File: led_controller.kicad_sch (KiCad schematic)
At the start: 33 parts, among them IC1 ESP32-C3-MINI-1-N4X, IC2 L6983N33QTR, J1 Screw_Terminal_01x02, J2 Screw_Terminal_01x02, J3 Conn_01x04_Pin, J4 Screw_Terminal_01x02, J5 Conn_01x03_Pin, Q2 FQD13N10LTM

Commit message: Add files via upload
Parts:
- R1, R2, R3, R4, R5, R6, R7: footprint Resistor_SMD:R_1206_3216Metric_Pad1.30x1.75mm_HandSolder -> Resistor_SMD:R_0805_2012Metric_Pad1.20x1.40mm_HandSolder
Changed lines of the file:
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@@
 			)
 		)
-		(property "Footprint" "Resistor_SMD:R_1206_3216Metric_Pad1.30x1.75mm_HandSolder"
+		(property "Footprint" "Resistor_SMD:R_0805_2012Metric_Pad1.20x1.40mm_HandSolder"
 			(at 33.02 118.618 90)
 			(effects
@@
 			)
 		)
-		(property "Footprint" "Resistor_SMD:R_1206_3216Metric_Pad1.30x1.75mm_HandSolder"
+		(property "Footprint" "Resistor_SMD:R_0805_2012Metric_Pad1.20x1.40mm_HandSolder"
 			(at 186.69 149.098 90)
 			(effects
@@
 			)
 		)
-		(property "Footprint" "Resistor_SMD:R_1206_3216Metric_Pad1.30x1.75mm_HandSolder"
+		(property "Footprint" "Resistor_SMD:R_0805_2012Metric_Pad1.20x1.40mm_HandSolder"
 			(at 31.75 145.288 90)
 			(effects
@@
 			)
 		)
-		(property "Footprint" "Resistor_SMD:R_1206_3216Metric_Pad1.30x1.75mm_HandSolder"
+		(property "Footprint" "Resistor_SMD:R_0805_2012Metric_Pad1.20x1.40mm_HandSolder"
 			(at 197.358 91.44 90)
 			(effects
@@
 			)
 		)
-		(property "Footprint" "Resistor_SMD:R_1206_3216Metric_Pad1.30x1.75mm_HandSolder"
+		(property "Footprint" "Resistor_SMD:R_0805_2012Metric_Pad1.20x1.40mm_HandSolder"
 			(at 191.77 89.408 90)
 			(effects
@@
 			)
 		)
-		(property "Footprint" "Resistor_SMD:R_1206_3216Metric_Pad1.30x1.75mm_HandSolder"
+		(property "Footprint" "Resistor_SMD:R_0805_2012Metric_Pad1.20x1.40mm_HandSolder"
 			(at 180.34 61.468 90)
 			(effects
@@
 			)
 		)
-		(property "Footprint" "Resistor_SMD:R_1206_3216Metric_Pad1.30x1.75mm_HandSolder"
+		(property "Footprint" "Resistor_SMD:R_0805_2012Metric_Pad1.20x1.40mm_HandSolder"
 			(at 186.69 138.938 90)
 			(effects

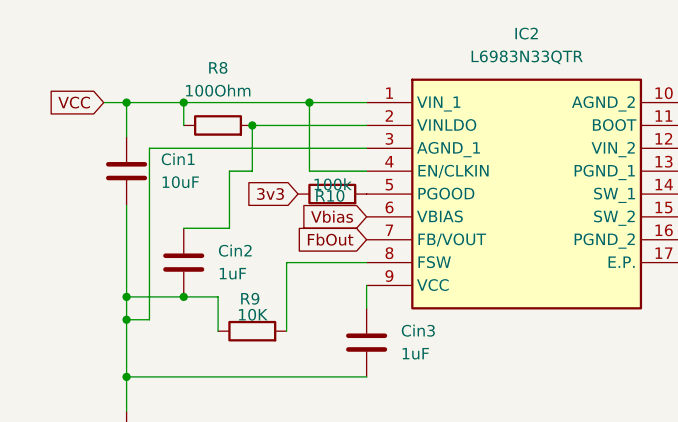
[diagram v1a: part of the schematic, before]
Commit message: Add files via upload
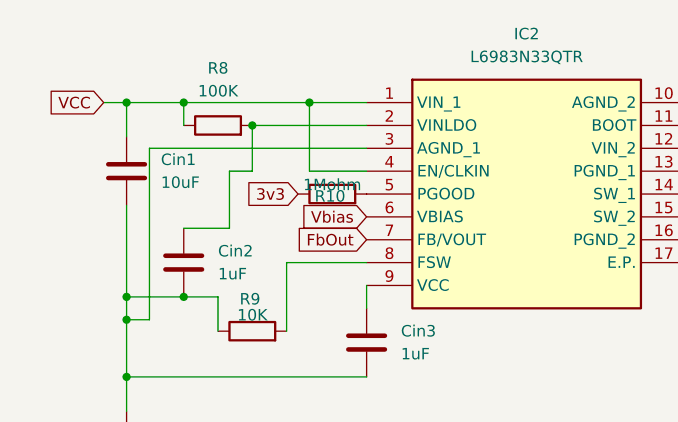
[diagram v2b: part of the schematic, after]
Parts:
- R10: value 100k -> 1Mohm
- R8: value 100Ohm -> 100K
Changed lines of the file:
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@@
 			)
 		)
-		(property "Value" "100Ohm"
+		(property "Value" "100K"
 			(at 43.18 27.94 90)
 			(effects
@@
 			)
 		)
-		(property "Value" "100k"
+		(property "Value" "1Mohm"
 			(at 55.88 38.354 90)
 			(effects
